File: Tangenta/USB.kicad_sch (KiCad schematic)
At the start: 12 parts, among them J12 907-211A1019D10200, J13 906-861A2116D10210, U8 USB2514B-I_M2

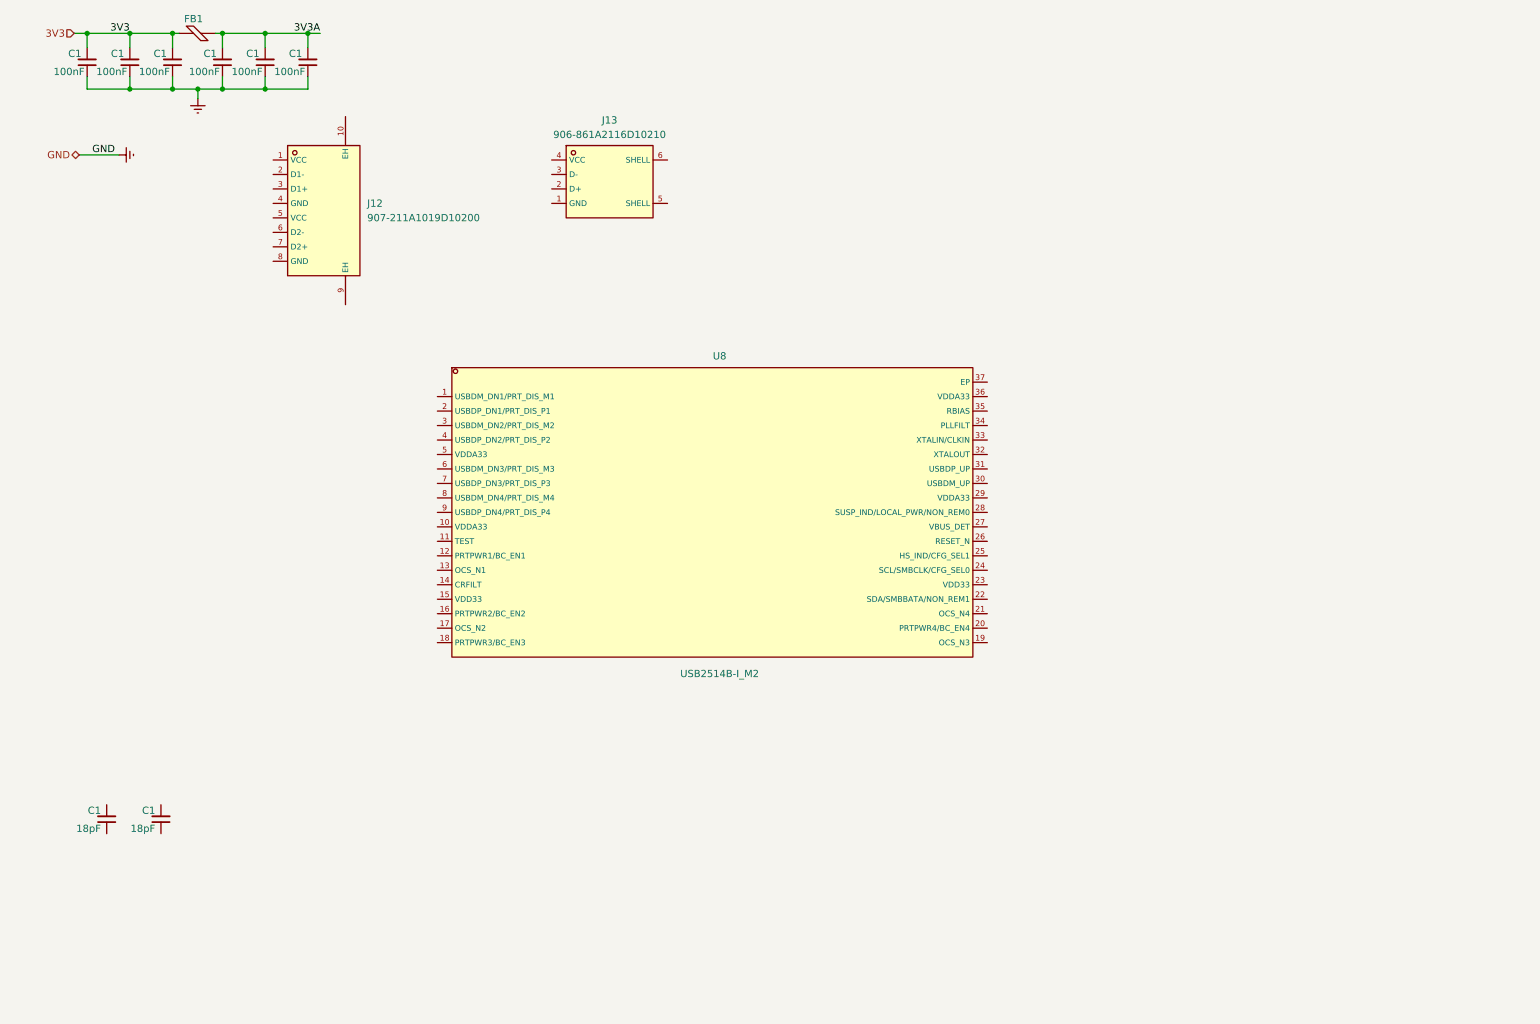
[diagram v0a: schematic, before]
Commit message: Current progress, USB...
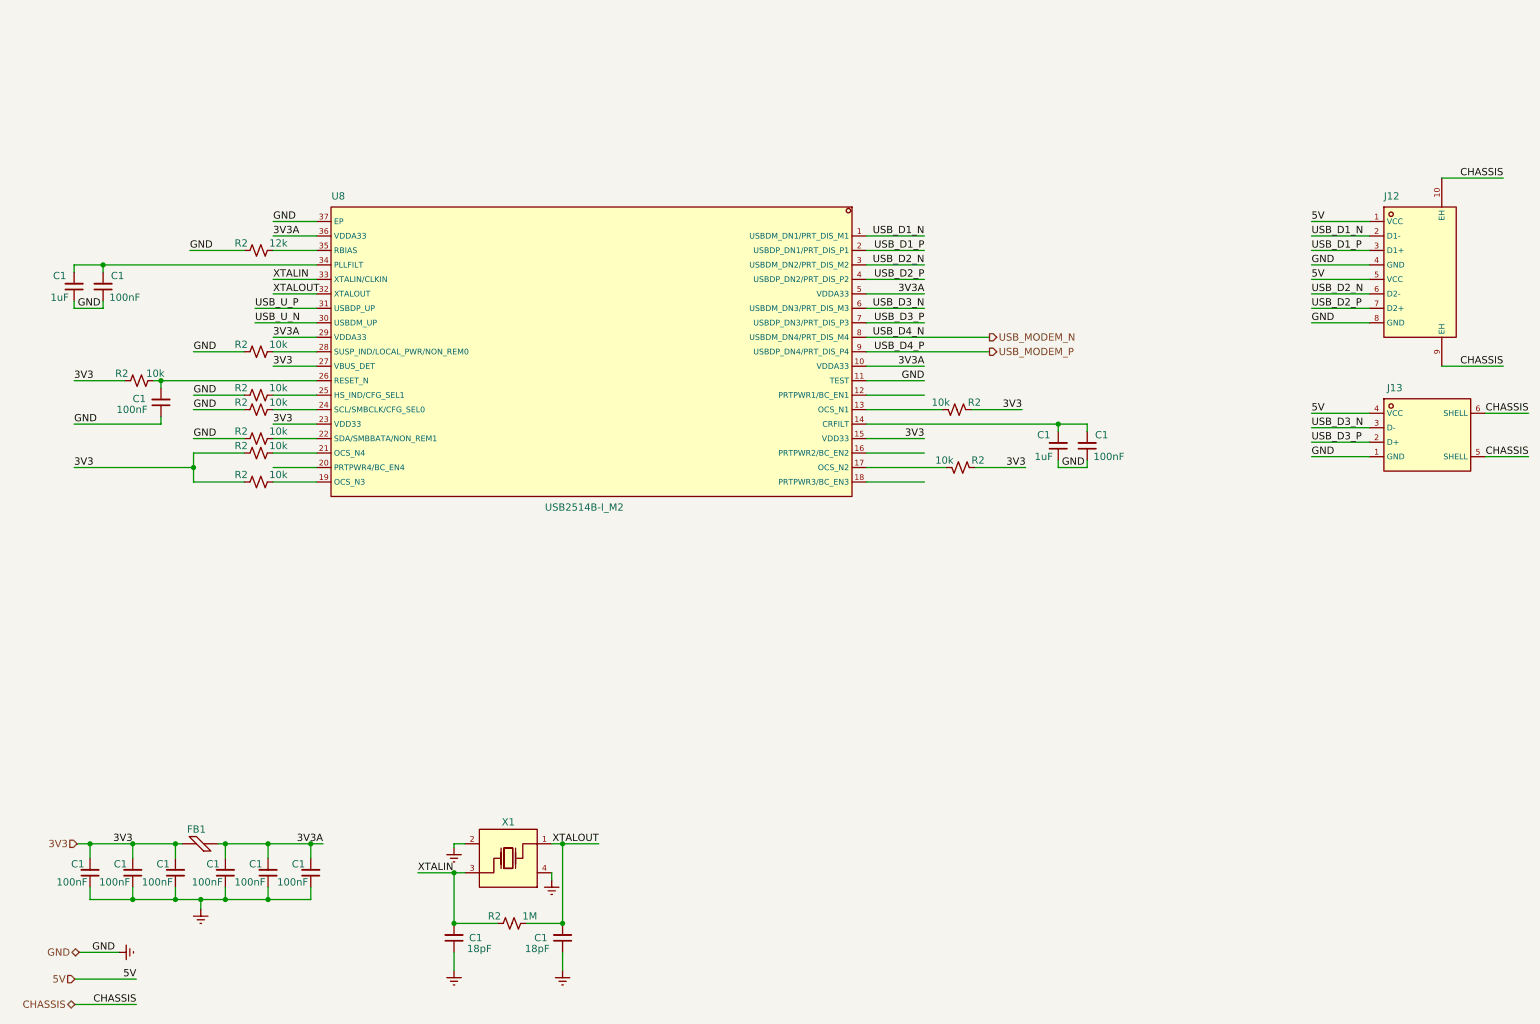
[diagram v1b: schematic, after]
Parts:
- added C1 (x3): 100nF, Capacitor_SMD:C_0402_1005Metric, symbol Device:C_Small
- added C1 (x2): 1uF, Capacitor_SMD:C_0402_1005Metric, symbol Device:C_Small
- added R2 (x9): 10k, Resistor_SMD:R_0402_1005Metric, symbol Device:R_Small_US
- added R2: 1M, Resistor_SMD:R_0402_1005Metric, symbol Device:R_Small_US
- added R2: 12k, Resistor_SMD:R_0402_1005Metric, symbol Device:R_Small_US
- added X1: X322524MOB4SI, XTAL_24MHZ:XTAL_24MHZ, symbol XTAL_24MHZ:X322524MOB4SI
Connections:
- net 3V3: now also U8.15 (VDD33), U8.23 (VDD33), U8.27 (VBUS_DET), R2.1, R2.1, R2.1, R2.1, R2.1
- net 3V3A: now also U8.10 (VDDA33), U8.29 (VDDA33), U8.36 (VDDA33), U8.5 (VDDA33)
- net GNDREF: now also C1.1, C1.1, U8.11 (TEST), U8.37 (EP), C1.1, C1.1, C1.1, C1.1, C1.1, R2.1, R2.1, R2.1, R2.1, R2.1, X1.2 (GND), X1.4 (GND)
- net XTALIN: now reaches C1.2
- net XTALIN: now also U8.33 (XTALIN/CLKIN), R2.1, X1.3 (OSC2)
- net USB_D1_N: now reaches U8.1 (USBDM_DN1/PRT_DIS_M1)
- net at U8.13 (OCS_N1): now also R2.2
- net at U8.14 (CRFILT): now also C1.2, C1.2
- net at U8.17 (OCS_N2): now also R2.2
- net at U8.19 (OCS_N3): now also R2.2
- net USB_D1_P: now reaches U8.2 (USBDP_DN1/PRT_DIS_P1)
- net at U8.21 (OCS_N4): now also R2.2
- net at U8.22 (SDA/SMBBATA/NON_REM1): now also R2.2
- net at U8.24 (SCL/SMBCLK/CFG_SEL0): now also R2.2
- net at U8.25 (HS_IND/CFG_SEL1): now also R2.2
- net at U8.26 (RESET_N): now also C1.2, R2.2
- net at U8.28 (SUSP_IND/LOCAL_PWR/NON_REM0): now also R2.2
- net USB_D2_N: now reaches U8.3 (USBDM_DN2/PRT_DIS_M2)
- net USB_U_N: now reaches U8.30 (USBDM_UP)
- net USB_U_P: now reaches U8.31 (USBDP_UP)
- net XTALOUT: now reaches U8.32 (XTALOUT)
- net XTALOUT: now also C1.2, R2.2, X1.1 (OSC1)
- net at U8.34 (PLLFILT): now also C1.2, C1.2
- net at U8.35 (RBIAS): now also R2.2
- net USB_D2_P: now reaches U8.4 (USBDP_DN2/PRT_DIS_P2)
- net USB_D3_N: now reaches U8.6 (USBDM_DN3/PRT_DIS_M3)
- net USB_D3_P: now reaches U8.7 (USBDP_DN3/PRT_DIS_P3)
- net USB_MODEM_N: now reaches U8.8 (USBDM_DN4/PRT_DIS_M4)
- net USB_MODEM_P: now reaches U8.9 (USBDP_DN4/PRT_DIS_P4)
- net CHASSIS: now reaches J13.5 (SHELL)
- net CHASSIS: now also J12.10 (EH), J12.9 (EH), J13.6 (SHELL)
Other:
- moved on the sheet: C1, FB1, J12, J13, U8
